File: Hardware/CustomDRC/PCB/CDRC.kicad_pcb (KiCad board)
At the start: 2 copper layers, 85 x 28.5 mm, 82 parts, among them IC301 SN65HVD75DR, J101 DSP Header, J401 TC2030NL - For UART PROG, J501 JST-PH-2.0-05, J502 JST-PH-2.0-02, J504 JST-PH-2.0-05, Q501 AO3400A, U201 AP63203WU-7, U401 ESP32-WROOM-32UE-R2, U501 ESD224DQA, U502 ESD224DQA

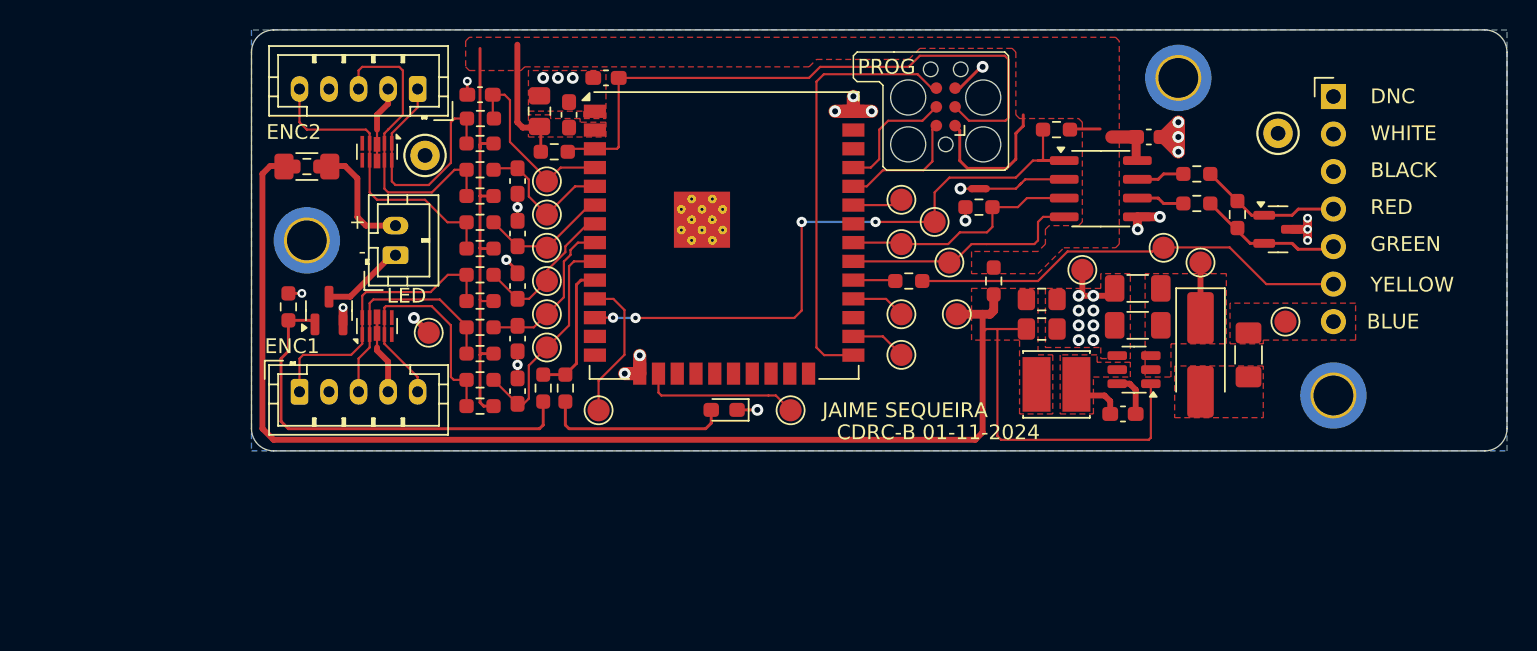
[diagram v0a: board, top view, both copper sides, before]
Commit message: Sync changes to Rev B HW
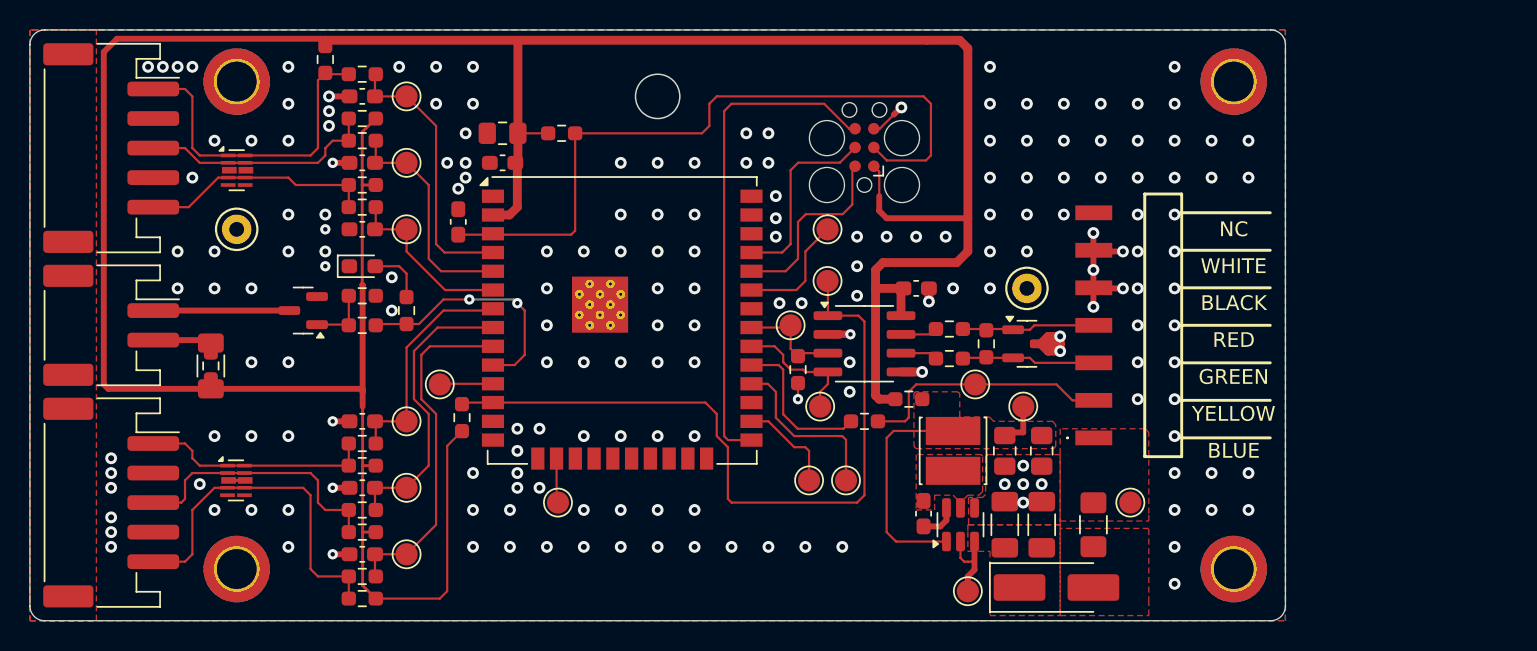
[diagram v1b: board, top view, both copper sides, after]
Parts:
- removed TP201, TP507: TestPoint_Small, TestPoint:TestPoint_Pad_D1.5mm
- added H104: MountingHole, MountingHole:MountingHole_2.7mm_M2.5_ISO7380_Pad_TopBottom, B.Cu at (190.0, 114.8)
- H101, H102, H103: footprint MountingHole:MountingHole_2.7mm_M2.5_ISO7380_Pad_TopOnly -> MountingHole:MountingHole_2.7mm_M2.5_ISO7380_Pad_TopBottom
- J101: footprint Connector_PinHeader_2.54mm:PinHeader_1x07_P2.54mm_Horizontal -> CDRC_Footprints:M208900705
- J501, J504: value JST-PH-2.0-05 -> JST_PH_S5B-PH-SM4; footprint Connector_JST:JST_PH_B5B-PH-K_1x05_P2.00mm_Vertical -> Connector_JST:JST_PH_S5B-PH-SM4-TB_1x05-1MP_P2.00mm_Horizontal
- J502: value JST-PH-2.0-02 -> ST_PH_S2B-PH-SM4; footprint Connector_JST:JST_PH_B2B-PH-K_1x02_P2.00mm_Vertical -> Connector_JST:JST_PH_S2B-PH-SM4-TB_1x02-1MP_P2.00mm_Horizontal
- moved H103 77.2 mm to (122.5, 81.8)
- moved H101 71.9 mm to (122.5, 114.8)
- moved H102 63.7 mm to (190.0, 81.8)
- moved R301 44.7 mm to (137.8, 104.5), turned to 90 degrees
- moved J501 34.9 mm to (114.0, 110.2), turned to -90 degrees
- moved TP204 27.3 mm to (172.0, 116.2)
- moved D401 26.4 mm to (131.0, 94.2), turned to 0 degrees
- moved J504 20.9 mm to (114.0, 86.2), turned to -90 degrees
- moved TP101 20.0 mm to (176.0, 95.8)
- moved J502 19.8 mm to (114.0, 98.2), turned to -90 degrees
- moved R302 19.8 mm to (170.8, 98.5)
- moved R304 19.8 mm to (170.8, 100.5)
- moved IC301 19.1 mm to (165.0, 99.5)
- moved R303 19.1 mm to (173.2, 99.5)
- moved C301 18.8 mm to (168.5, 95.8)
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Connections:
- J101 pad 1: unconnected-(J101-Pin_1-Pad1) -> /DSP_CONST_12V
- J101 pad 2: GND -> /DSP_POWER_EN
- J101 pad 3: GND -> /DSP_RS485_A/Y
- J101 pad 5: /DSP_RS485_A/Y -> GND
- J101 pad 6: /DSP_POWER_EN -> GND
- J101 pad 7: /DSP_CONST_12V -> unconnected-(J101-Pin_7-Pad7)
- J501 pad 1: /USER_INTERFACE/ENC_2_A -> /USER_INTERFACE/ENC_1_A
- J501 pad 3: /USER_INTERFACE/ENC_2_B -> /USER_INTERFACE/ENC_1_B
- J501 pad 5: /USER_INTERFACE/ENC_2_SW -> /USER_INTERFACE/ENC_1_SW
- J504 pad 1: /USER_INTERFACE/ENC_1_A -> /USER_INTERFACE/ENC_2_A
- J504 pad 3: /USER_INTERFACE/ENC_1_B -> /USER_INTERFACE/ENC_2_B
- J504 pad 5: /USER_INTERFACE/ENC_1_SW -> /USER_INTERFACE/ENC_2_SW
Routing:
- net VCC: track 168.5 -> 237.1 mm
- net Net-(Q501-G): track 28.6 -> 4.10 mm
- net GND: track 45.8 -> 27.1 mm, vias 35 -> 192
- net /DSP_POWER_EN: track 29.3 -> 17.1 mm
- net /MCU/IO19: track 16.4 -> 6.62 mm
- net /MCU/IO32: track 10.9 -> 19.9 mm
- net Net-(D401-A): track 12.6 -> 3.92 mm
- net /MCU/IO33: track 14.8 -> 23.4 mm
- net Net-(U401-IO17): track 3.68 -> 11.7 mm
- net Net-(U401-IO13): track 10.7 -> 2.89 mm
- net /MCU/IO18: track 16.5 -> 8.75 mm
- net /MCU/DSP_EN: track 2.86 -> 10.5 mm
- net /MCU/IO25: track 9.28 -> 16.4 mm, vias 0 -> 2
- net Net-(U401-IO26): track 9.83 -> 3.56 mm
- net /MCU/IO39: track 9.52 -> 15.4 mm
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- added copper zone on F.Cu, net /USER_INTERFACE/MNT
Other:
- board size 85 x 28.5 mm -> 85 x 40 mm
- board text added: "ANT"
- board text added: "ENC_1A"
- board text added: "ENC_1B"
- board text added: "ENC_1SW"
- board text added: "ENC_2A"
- board text added: "ENC_2B"
- board text added: "ENC_2SW"
- board text added: "NC"
- board text removed: "+"
- board text removed: "-"
- board text removed: "12V BLUE"
- board text removed: "1A"
- board text removed: "1B"
- board text removed: "1SW"
- board text removed: "2A"
- board text removed: "2B"
- board text removed: "2SW"
- board text removed: "A/Y GREEN"
- board text removed: "B/Z RED"
- board text removed: "DNC"
- board text removed: "ENC1"
- board text removed: "ENC2"
- board text removed: "GND BLACK"
- board text removed: "GND WHITE"
- board text removed: "GND YELLOW"
- board text removed: "LED"
- board text removed: "MNT"
- board text removed: "PROG"
